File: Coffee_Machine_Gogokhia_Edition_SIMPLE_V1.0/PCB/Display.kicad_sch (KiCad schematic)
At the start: 2 parts

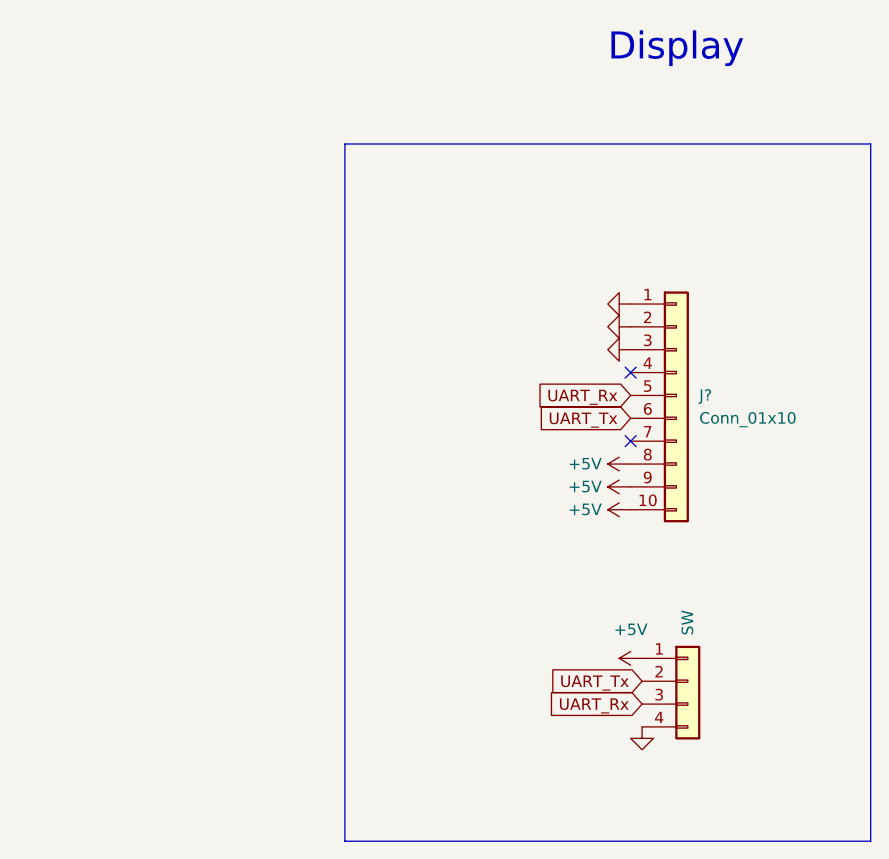
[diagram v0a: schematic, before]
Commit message: Edited
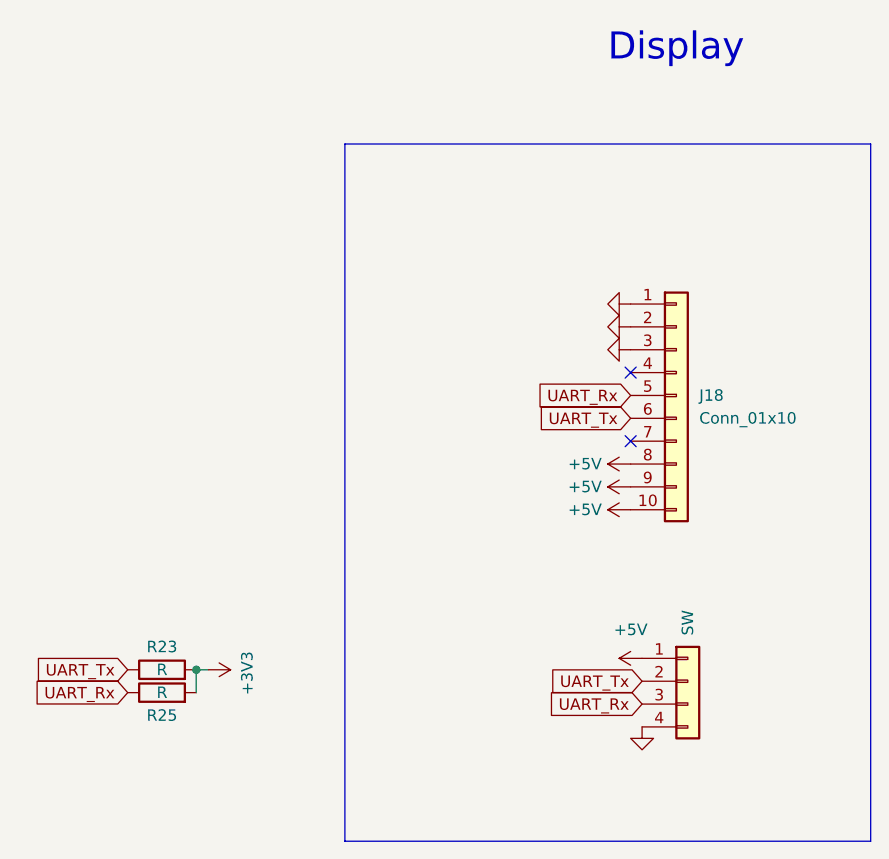
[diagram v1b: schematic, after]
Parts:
- added R23, R25: R, Resistor_SMD:R_0603_1608Metric, symbol Device:R
- J18: renamed from J?; footprint (none) -> Footprint:FCC_1.0mm_10P
- J19: renamed from J?; footprint Connector_PinHeader_1.27mm:PinHeader_1x04_P1.27mm_Vertical -> Footprint:XH2.54_4P_SMD
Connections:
- net UART_Rx: now also R25.1
- net UART_Tx: now also R23.1
- new net +3V3: R23.2, R25.2
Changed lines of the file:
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@@
 (kicad_sch (version 20211123) (generator eeschema)
   (paper "A4")
+  (junction (at 58.42 123.19) (diameter 0) (color 0 0 0 0)
+  )
   (no_connect (at 106.68 97.79))
   (no_connect (at 106.68 90.17))
@@
     (stroke (width 0) (type default) (color 0 0 0 0))
   )
+  (wire (pts (xy 58.42 123.19) (xy 59.69 123.19))
+    (stroke (width 0) (type default) (color 0 0 0 0))
+  )
   (polyline (pts (xy 74.93 64.77) (xy 133.35 64.77))
     (stroke (width 0) (type default) (color 0 0 0 0))
@@
   )
   (polyline (pts (xy 133.35 64.77) (xy 133.35 142.24))
+    (stroke (width 0) (type default) (color 0 0 0 0))
+  )
+  (wire (pts (xy 58.42 123.19) (xy 58.42 125.73))
     (stroke (width 0) (type default) (color 0 0 0 0))
   )
@@
     )
   )
+  (global_label "UART_Tx" (shape input) (at 50.8 123.19 180) (fields_autoplaced)
+    (effects (font (size 1.27 1.27)) (justify right))
+    (property "Intersheet References" "${INTERSHEET_REFS}" (id 0) (at 40.8558 123.2694 0)
+      (effects (font (size 1.27 1.27)) (justify right) hide)
+    )
+  )
   (global_label "UART_Tx" (shape input) (at 107.95 124.46 180) (fields_autoplaced)
     (effects (font (size 1.27 1.27)) (justify right))
@@
     )
   )
+  (global_label "UART_Rx" (shape input) (at 50.8 125.73 180) (fields_autoplaced)
+    (effects (font (size 1.27 1.27)) (justify right))
+    (property "Intersheet References" "${INTERSHEET_REFS}" (id 0) (at 40.5534 125.8094 0)
+      (effects (font (size 1.27 1.27)) (justify right) hide)
+    )
+  )
   (global_label "UART_Rx" (shape input) (at 106.68 92.71 180) (fields_autoplaced)
     (effects (font (size 1.27 1.27)) (justify right))
@@
   (symbol (lib_id "power:+5V") (at 106.68 100.33 90) (unit 1)
     (in_bom yes) (on_board yes)
-    (property "Reference" "#PWR?" (id 0) (at 110.49 100.33 0)
+    (property "Reference" "#PWR0159" (id 0) (at 110.49 100.33 0)
       (effects (font (size 1.27 1.27)) hide)
     )
@@
     (pin "1")
   )
+  (symbol (lib_id "Device:R") (at 54.61 123.19 90) (unit 1)
+    (in_bom yes) (on_board yes)
+    (property "Reference" "R23" (id 0) (at 54.61 120.65 90))
+    (property "Value" "R" (id 1) (at 54.61 123.19 90))
+    (property "Footprint" "Resistor_SMD:R_0603_1608Metric" (id 2) (at 54.61 124.968 90)
+      (effects (font (size 1.27 1.27)) hide)
+    )
+    (property "Datasheet" "~" (id 3) (at 54.61 123.19 0)
+      (effects (font (size 1.27 1.27)) hide)
+    )
+    (pin "1")
+    (pin "2")
+  )
+  (symbol (lib_id "power:+3V3") (at 59.69 123.19 270) (unit 1)
+    (in_bom yes) (on_board yes)
+    (property "Reference" "#PWR0163" (id 0) (at 55.88 123.19 0)
+      (effects (font (size 1.27 1.27)) hide)
+    )
+    (property "Value" "+3V3" (id 1) (at 64.0842 123.571 0))
+    (property "Footprint" "" (id 2) (at 59.69 123.19 0)
+      (effects (font (size 1.27 1.27)) hide)
+    )
+    (property "Datasheet" "" (id 3) (at 59.69 123.19 0)
+      (effects (font (size 1.27 1.27)) hide)
+    )
+    (pin "1")
+  )
   (symbol (lib_id "power:+5V") (at 106.68 102.87 90) (unit 1)
     (in_bom yes) (on_board yes)
-    (property "Reference" "#PWR?" (id 0) (at 110.49 102.87 0)
+    (property "Reference" "#PWR0156" (id 0) (at 110.49 102.87 0)
       (effects (font (size 1.27 1.27)) hide)
     )
@@
   (symbol (lib_id "power:GND") (at 107.95 129.54 0) (unit 1)
     (in_bom yes) (on_board yes)
-    (property "Reference" "#PWR?" (id 0) (at 107.95 135.89 0)
+    (property "Reference" "#PWR0154" (id 0) (at 107.95 135.89 0)
       (effects (font (size 1.27 1.27)) hide)
     )
@@
   (symbol (lib_id "power:GND") (at 106.68 87.63 270) (unit 1)
     (in_bom yes) (on_board yes)
-    (property "Reference" "#PWR?" (id 0) (at 100.33 87.63 0)
+    (property "Reference" "#PWR0158" (id 0) (at 100.33 87.63 0)
       (effects (font (size 1.27 1.27)) hide)
     )
@@
   (symbol (lib_id "power:GND") (at 106.68 82.55 270) (unit 1)
     (in_bom yes) (on_board yes)
-    (property "Reference" "#PWR?" (id 0) (at 100.33 82.55 0)
+    (property "Reference" "#PWR0157" (id 0) (at 100.33 82.55 0)
       (effects (font (size 1.27 1.27)) hide)
     )
@@
   (symbol (lib_id "power:+5V") (at 106.68 105.41 90) (unit 1)
     (in_bom yes) (on_board yes)
-    (property "Reference" "#PWR?" (id 0) (at 110.49 105.41 0)
+    (property "Reference" "#PWR0155" (id 0) (at 110.49 105.41 0)
       (effects (font (size 1.27 1.27)) hide)
     )
@@
   (symbol (lib_id "Connector_Generic:Conn_01x10") (at 111.76 92.71 0) (unit 1)
     (in_bom yes) (on_board yes) (fields_autoplaced)
-    (property "Reference" "J?" (id 0) (at 114.3 92.7099 0)
+    (property "Reference" "J18" (id 0) (at 114.3 92.7099 0)
       (effects (font (size 1.27 1.27)) (justify left))
     )
@@
       (effects (font (size 1.27 1.27)) (justify left))
     )
-    (property "Footprint" "" (id 2) (at 111.76 92.71 0)
+    (property "Footprint" "Footprint:FCC_1.0mm_10P" (id 2) (at 111.76 92.71 0)
       (effects (font (size 1.27 1.27)) hide)
     )
@@
   (symbol (lib_id "power:+5V") (at 107.95 121.92 90) (unit 1)
     (in_bom yes) (on_board yes)
-    (property "Reference" "#PWR?" (id 0) (at 111.76 121.92 0)
+    (property "Reference" "#PWR0153" (id 0) (at 111.76 121.92 0)
       (effects (font (size 1.27 1.27)) hide)
     )
@@
   (symbol (lib_id "power:GND") (at 106.68 85.09 270) (unit 1)
     (in_bom yes) (on_board yes)
-    (property "Reference" "#PWR?" (id 0) (at 100.33 85.09 0)
+    (property "Reference" "#PWR0160" (id 0) (at 100.33 85.09 0)
       (effects (font (size 1.27 1.27)) hide)
     )
@@
   (symbol (lib_id "Connector_Generic:Conn_01x04") (at 113.03 124.46 0) (unit 1)
     (in_bom yes) (on_board yes)
-    (property "Reference" "J?" (id 0) (at 115.062 124.6632 0)
+    (property "Reference" "J19" (id 0) (at 115.062 124.6632 0)
       (effects (font (size 1.27 1.27)) (justify left) hide)
     )
@@
       (effects (font (size 1.27 1.27)) (justify left))
     )
-    (property "Footprint" "Connector_PinHeader_1.27mm:PinHeader_1x04_P1.27mm_Vertical" (id 2) (at 113.03 124.46 0)
+    (property "Footprint" "Footprint:XH2.54_4P_SMD" (id 2) (at 113.03 124.46 0)
       (effects (font (size 1.27 1.27)) hide)
     )
@@
     (pin "4")
   )
+  (symbol (lib_id "Device:R") (at 54.61 125.73 90) (unit 1)
+    (in_bom yes) (on_board yes)
+    (property "Reference" "R25" (id 0) (at 54.61 128.27 90))
+    (property "Value" "R" (id 1) (at 54.61 125.73 90))
+    (property "Footprint" "Resistor_SMD:R_0603_1608Metric" (id 2) (at 54.61 127.508 90)
+      (effects (font (size 1.27 1.27)) hide)
+    )
+    (property "Datasheet" "~" (id 3) (at 54.61 125.73 0)
+      (effects (font (size 1.27 1.27)) hide)
+    )
+    (pin "1")
+    (pin "2")
+  )
 )

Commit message: 1
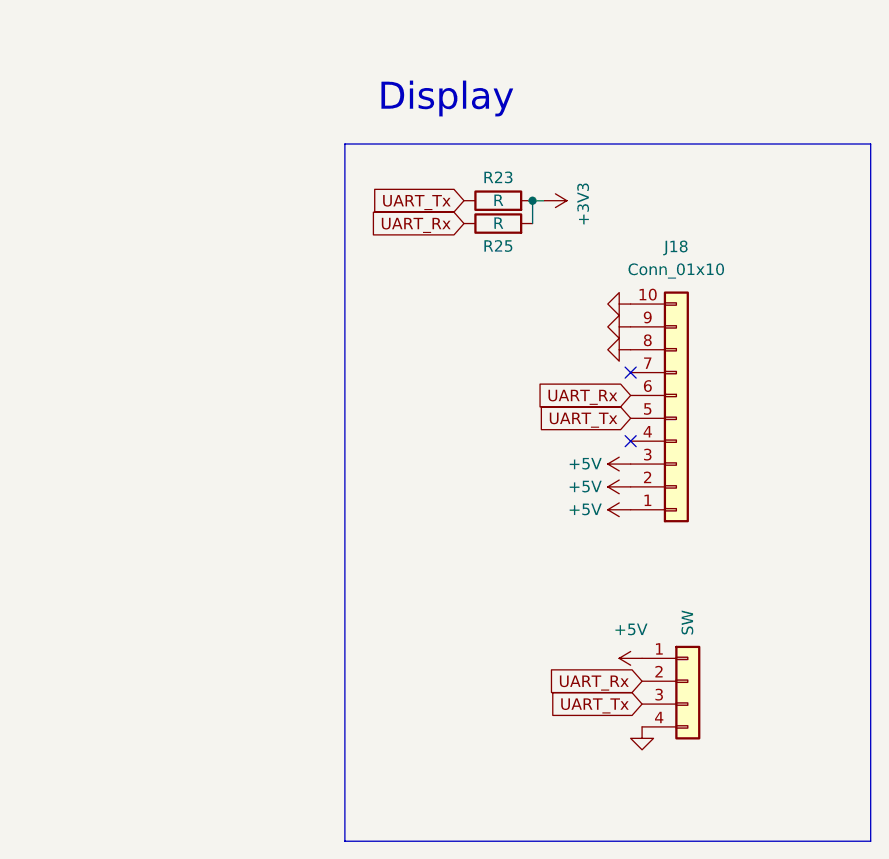
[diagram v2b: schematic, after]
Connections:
- net +5V: now also J18.1 (Pin_1), J18.2 (Pin_2), J18.3 (Pin_3); no longer J18.10 (Pin_10), J18.8 (Pin_8), J18.9 (Pin_9)
- net GND: now also J18.10 (Pin_10), J18.8 (Pin_8), J18.9 (Pin_9); no longer J18.1 (Pin_1), J18.2 (Pin_2), J18.3 (Pin_3)
- net UART_Rx: now also J18.6 (Pin_6), J19.2 (Pin_2); no longer J18.5 (Pin_5), J19.3 (Pin_3)
- net UART_Tx: now also J18.5 (Pin_5), J19.3 (Pin_3); no longer J18.6 (Pin_6), J19.2 (Pin_2)
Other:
- moved on the sheet: R23, R25
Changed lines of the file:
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@@
 (kicad_sch (version 20211123) (generator eeschema)
   (paper "A4")
-  (junction (at 58.42 123.19) (diameter 0) (color 0 0 0 0)
+  (junction (at 95.7834 71.0692) (diameter 0) (color 0 0 0 0)
   )
   (no_connect (at 106.68 97.79))
@@
     (stroke (width 0) (type default) (color 0 0 0 0))
   )
-  (wire (pts (xy 58.42 123.19) (xy 59.69 123.19))
+  (wire (pts (xy 95.7834 71.0692) (xy 97.0534 71.0692))
     (stroke (width 0) (type default) (color 0 0 0 0))
   )
@@
     (stroke (width 0) (type default) (color 0 0 0 0))
   )
-  (wire (pts (xy 58.42 123.19) (xy 58.42 125.73))
-    (stroke (width 0) (type default) (color 0 0 0 0))
-  )
-  (text "Display" (at 104.14 55.88 0)
+  (wire (pts (xy 95.7834 71.0692) (xy 95.7834 73.6092))
+    (stroke (width 0) (type default) (color 0 0 0 0))
+  )
+  (text "Display" (at 78.5876 61.468 0)
     (effects (font (size 3 3)) (justify left bottom))
   )
@@
     )
   )
-  (global_label "UART_Tx" (shape input) (at 50.8 123.19 180) (fields_autoplaced)
-    (effects (font (size 1.27 1.27)) (justify right))
-    (property "Intersheet References" "${INTERSHEET_REFS}" (id 0) (at 40.8558 123.2694 0)
-      (effects (font (size 1.27 1.27)) (justify right) hide)
-    )
-  )
-  (global_label "UART_Tx" (shape input) (at 107.95 124.46 180) (fields_autoplaced)
-    (effects (font (size 1.27 1.27)) (justify right))
-    (property "Intersheet References" "${INTERSHEET_REFS}" (id 0) (at 98.0058 124.5394 0)
-      (effects (font (size 1.27 1.27)) (justify right) hide)
-    )
-  )
-  (global_label "UART_Rx" (shape input) (at 107.95 127 180) (fields_autoplaced)
-    (effects (font (size 1.27 1.27)) (justify right))
-    (property "Intersheet References" "${INTERSHEET_REFS}" (id 0) (at 97.7034 127.0794 0)
-      (effects (font (size 1.27 1.27)) (justify right) hide)
-    )
-  )
-  (global_label "UART_Rx" (shape input) (at 50.8 125.73 180) (fields_autoplaced)
-    (effects (font (size 1.27 1.27)) (justify right))
-    (property "Intersheet References" "${INTERSHEET_REFS}" (id 0) (at 40.5534 125.8094 0)
+  (global_label "UART_Tx" (shape input) (at 88.1634 71.0692 180) (fields_autoplaced)
+    (effects (font (size 1.27 1.27)) (justify right))
+    (property "Intersheet References" "${INTERSHEET_REFS}" (id 0) (at 78.2192 71.1486 0)
+      (effects (font (size 1.27 1.27)) (justify right) hide)
+    )
+  )
+  (global_label "UART_Tx" (shape input) (at 107.95 127 180) (fields_autoplaced)
+    (effects (font (size 1.27 1.27)) (justify right))
+    (property "Intersheet References" "${INTERSHEET_REFS}" (id 0) (at 98.0058 127.0794 0)
+      (effects (font (size 1.27 1.27)) (justify right) hide)
+    )
+  )
+  (global_label "UART_Rx" (shape input) (at 107.95 124.46 180) (fields_autoplaced)
+    (effects (font (size 1.27 1.27)) (justify right))
+    (property "Intersheet References" "${INTERSHEET_REFS}" (id 0) (at 97.7034 124.5394 0)
+      (effects (font (size 1.27 1.27)) (justify right) hide)
+    )
+  )
+  (global_label "UART_Rx" (shape input) (at 88.1634 73.6092 180) (fields_autoplaced)
+    (effects (font (size 1.27 1.27)) (justify right))
+    (property "Intersheet References" "${INTERSHEET_REFS}" (id 0) (at 77.9168 73.6886 0)
       (effects (font (size 1.27 1.27)) (justify right) hide)
     )
@@
     (pin "1")
   )
-  (symbol (lib_id "Device:R") (at 54.61 123.19 90) (unit 1)
-    (in_bom yes) (on_board yes)
-    (property "Reference" "R23" (id 0) (at 54.61 120.65 90))
-    (property "Value" "R" (id 1) (at 54.61 123.19 90))
-    (property "Footprint" "Resistor_SMD:R_0603_1608Metric" (id 2) (at 54.61 124.968 90)
-      (effects (font (size 1.27 1.27)) hide)
-    )
-    (property "Datasheet" "~" (id 3) (at 54.61 123.19 0)
+  (symbol (lib_id "Device:R") (at 91.9734 71.0692 90) (unit 1)
+    (in_bom yes) (on_board yes)
+    (property "Reference" "R23" (id 0) (at 91.9734 68.5292 90))
+    (property "Value" "R" (id 1) (at 91.9734 71.0692 90))
+    (property "Footprint" "Resistor_SMD:R_0603_1608Metric" (id 2) (at 91.9734 72.8472 90)
+      (effects (font (size 1.27 1.27)) hide)
+    )
+    (property "Datasheet" "~" (id 3) (at 91.9734 71.0692 0)
       (effects (font (size 1.27 1.27)) hide)
     )
@@
     (pin "2")
   )
-  (symbol (lib_id "power:+3V3") (at 59.69 123.19 270) (unit 1)
-    (in_bom yes) (on_board yes)
-    (property "Reference" "#PWR0163" (id 0) (at 55.88 123.19 0)
-      (effects (font (size 1.27 1.27)) hide)
-    )
-    (property "Value" "+3V3" (id 1) (at 64.0842 123.571 0))
-    (property "Footprint" "" (id 2) (at 59.69 123.19 0)
-      (effects (font (size 1.27 1.27)) hide)
-    )
-    (property "Datasheet" "" (id 3) (at 59.69 123.19 0)
+  (symbol (lib_id "power:+3V3") (at 97.0534 71.0692 270) (unit 1)
+    (in_bom yes) (on_board yes)
+    (property "Reference" "#PWR0163" (id 0) (at 93.2434 71.0692 0)
+      (effects (font (size 1.27 1.27)) hide)
+    )
+    (property "Value" "+3V3" (id 1) (at 101.4476 71.4502 0))
+    (property "Footprint" "" (id 2) (at 97.0534 71.0692 0)
+      (effects (font (size 1.27 1.27)) hide)
+    )
+    (property "Datasheet" "" (id 3) (at 97.0534 71.0692 0)
       (effects (font (size 1.27 1.27)) hide)
     )
@@
     (pin "1")
   )
-  (symbol (lib_id "Connector_Generic:Conn_01x10") (at 111.76 92.71 0) (unit 1)
+  (symbol (lib_id "Connector_Generic:Conn_01x10") (at 111.76 95.25 0) (mirror x) (unit 1)
     (in_bom yes) (on_board yes) (fields_autoplaced)
-    (property "Reference" "J18" (id 0) (at 114.3 92.7099 0)
-      (effects (font (size 1.27 1.27)) (justify left))
-    )
-    (property "Value" "Conn_01x10" (id 1) (at 114.3 95.2499 0)
-      (effects (font (size 1.27 1.27)) (justify left))
-    )
-    (property "Footprint" "Footprint:FCC_1.0mm_10P" (id 2) (at 111.76 92.71 0)
-      (effects (font (size 1.27 1.27)) hide)
-    )
-    (property "Datasheet" "~" (id 3) (at 111.76 92.71 0)
+    (property "Reference" "J18" (id 0) (at 111.76 76.2 0))
+    (property "Value" "Conn_01x10" (id 1) (at 111.76 78.74 0))
+    (property "Footprint" "Footprint:FCC_1.0mm_10P" (id 2) (at 111.76 95.25 0)
+      (effects (font (size 1.27 1.27)) hide)
+    )
+    (property "Datasheet" "~" (id 3) (at 111.76 95.25 0)
       (effects (font (size 1.27 1.27)) hide)
     )
@@
     (pin "4")
   )
-  (symbol (lib_id "Device:R") (at 54.61 125.73 90) (unit 1)
-    (in_bom yes) (on_board yes)
-    (property "Reference" "R25" (id 0) (at 54.61 128.27 90))
-    (property "Value" "R" (id 1) (at 54.61 125.73 90))
-    (property "Footprint" "Resistor_SMD:R_0603_1608Metric" (id 2) (at 54.61 127.508 90)
-      (effects (font (size 1.27 1.27)) hide)
-    )
-    (property "Datasheet" "~" (id 3) (at 54.61 125.73 0)
-      (effects (font (size 1.27 1.27)) hide)
-    )
+  (symbol (lib_id "Device:R") (at 91.9734 73.6092 90) (unit 1)
+    (in_bom yes) (on_board yes)
+    (property "Reference" "R25" (id 0) (at 91.9734 76.1492 90))
+    (property "Value" "R" (id 1) (at 91.9734 73.6092 90))
+    (property "Footprint" "Resistor_SMD:R_0603_1608Metric" (id 2) (at 91.9734 75.3872 90)
+      (effects (font (size 1.27 1.27)) hide)
+    )
+    (property "Datasheet" "~" (id 3) (at 91.9734 73.6092 0)
+      (effects (font (size 1.27 1.27)) hide)
+    )
